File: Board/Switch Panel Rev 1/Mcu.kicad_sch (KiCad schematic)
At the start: 26 parts, among them J4 Conn_ARM_SWD_TagConnect_TC203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, J4 USB_C_Receptacle_USB2.0, U17 STM32G491CEUx, U6 MB85RS64, Y2 32.768kHz, Y3 8MHz

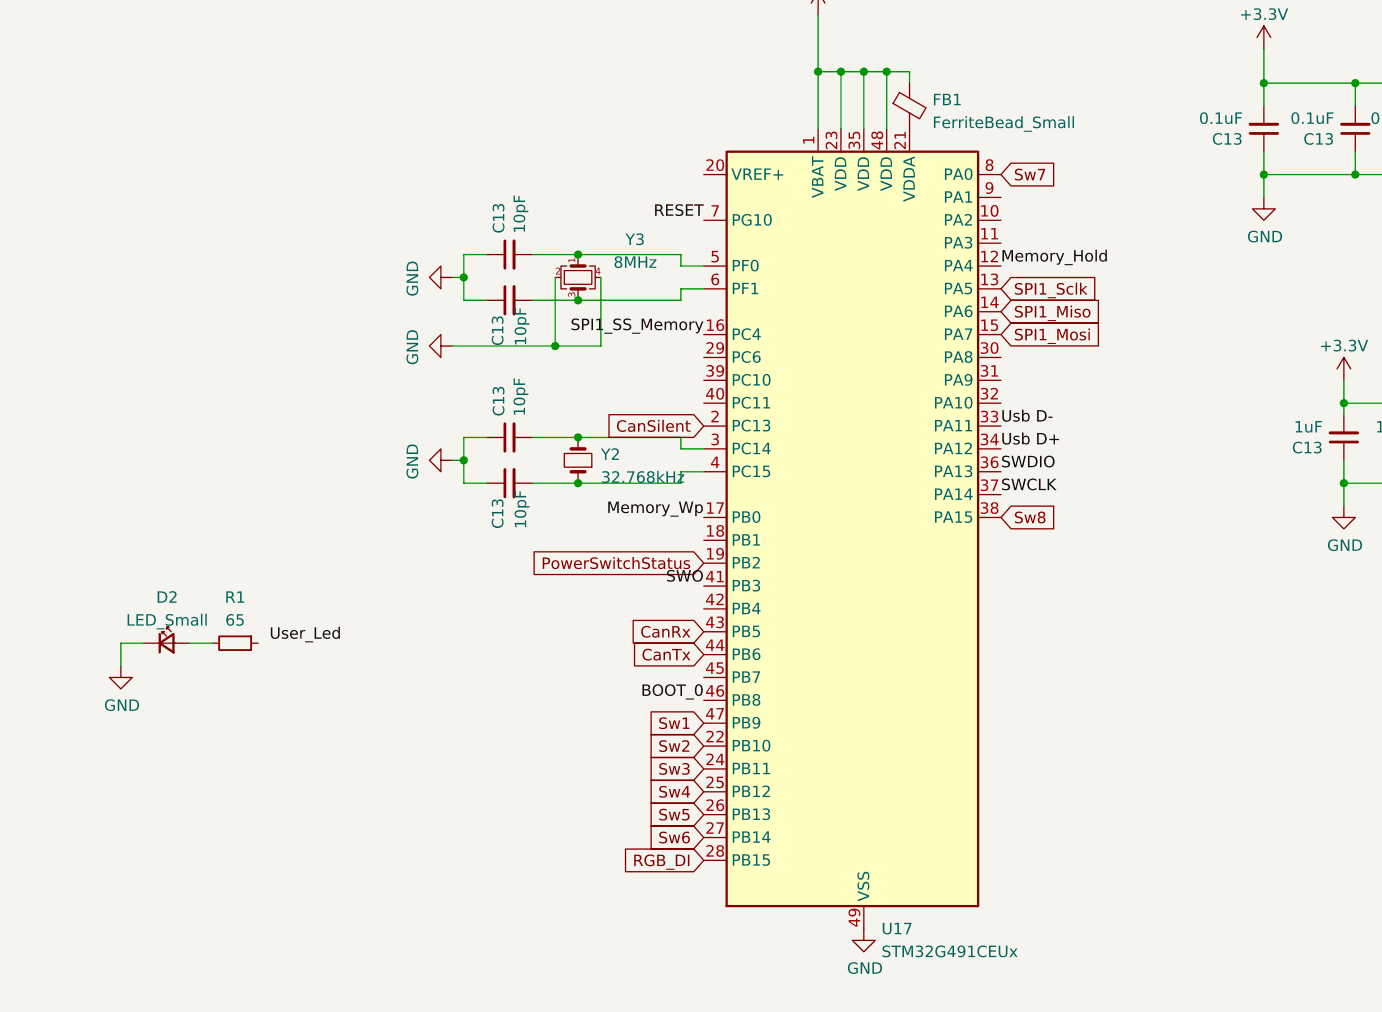
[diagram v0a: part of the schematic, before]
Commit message: Board Updates
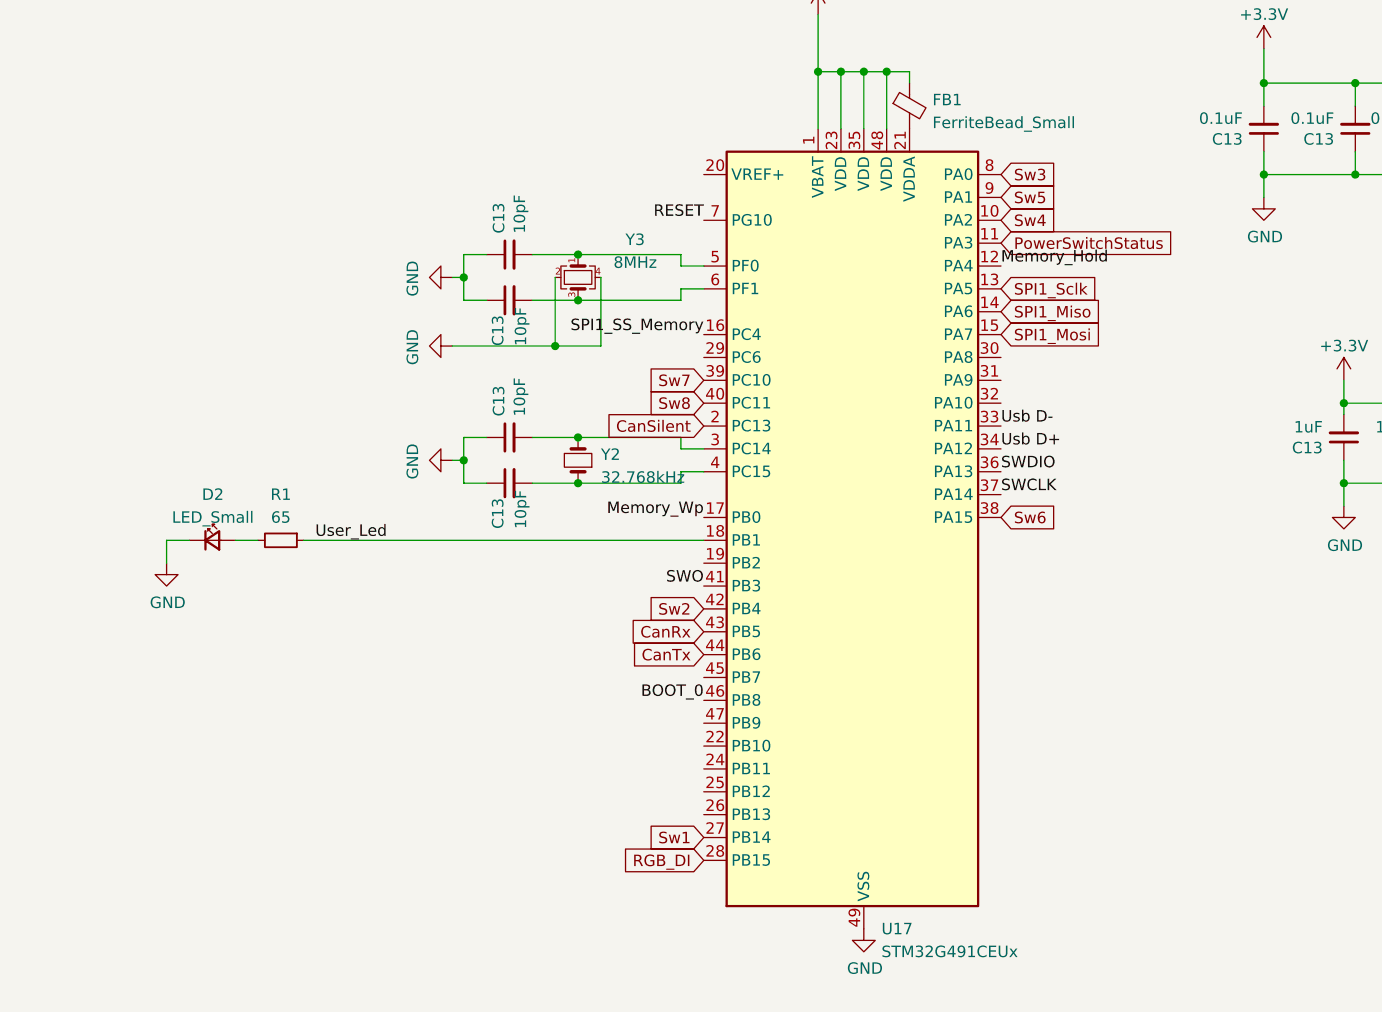
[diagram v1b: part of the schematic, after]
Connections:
- net PowerSwitchStatus: now also U17.11 (PA3); no longer U17.19 (PB2)
- net Sw1: now also U17.27 (PB14); no longer U17.47 (PB9)
- net Sw2: now also U17.42 (PB4); no longer U17.22 (PB10)
- net Sw3: now also U17.8 (PA0); no longer U17.24 (PB11)
- net Sw4: now also U17.10 (PA2); no longer U17.25 (PB12)
- net Sw5: now also U17.9 (PA1); no longer U17.26 (PB13)
- net Sw6: now also U17.38 (PA15); no longer U17.27 (PB14)
- net Sw7: now also U17.39 (PC10); no longer U17.8 (PA0)
- net Sw8: now also U17.40 (PC11); no longer U17.38 (PA15)
- net User_Led: now also R1.1, U17.18 (PB1)
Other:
- moved on the sheet: D2, R1
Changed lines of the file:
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@@
+    (stroke (width 0) (type default))
+  )
+  (wire (pts (xy 40.64 81.28) (xy 85.09 81.28))
     (stroke (width 0) (type default))
   )
@@
     (stroke (width 0) (type default))
   )
-  (wire (pts (xy 22.86 92.71) (xy 20.32 92.71))
+  (wire (pts (xy 27.94 81.28) (xy 25.4 81.28))
     (stroke (width 0) (type default))
   )
@@
     (stroke (width 0) (type default))
   )
-  (wire (pts (xy 27.94 92.71) (xy 30.48 92.71))
+  (wire (pts (xy 33.02 81.28) (xy 35.56 81.28))
     (stroke (width 0) (type default))
   )
@@
     (stroke (width 0) (type default))
   )
-  (wire (pts (xy 20.32 92.71) (xy 20.32 95.25))
+  (wire (pts (xy 25.4 81.28) (xy 25.4 83.82))
     (stroke (width 0) (type default))
   )
@@
     (effects (font (size 1.27 1.27)) (justify right bottom))
   )
-  (label "User_Led" (at 36.83 92.71 0) (fields_autoplaced)
+  (label "User_Led" (at 41.91 81.28 0) (fields_autoplaced)
     (effects (font (size 1.27 1.27)) (justify left bottom))
   )
@@
     (effects (font (size 1.27 1.27)) (justify right bottom))
   )
-  (global_label "Sw8" (shape input) (at 118.11 78.74 0) (fields_autoplaced)
-    (effects (font (size 1.27 1.27)) (justify left))
-    (property "Intersheetrefs" "${INTERSHEET_REFS}" (at 124.7653 78.74 0)
-      (effects (font (size 1.27 1.27)) (justify left) hide)
+  (global_label "Sw8" (shape input) (at 85.09 66.04 180) (fields_autoplaced)
+    (effects (font (size 1.27 1.27)) (justify right))
+    (property "Intersheetrefs" "${INTERSHEET_REFS}" (at 78.4347 66.04 0)
+      (effects (font (size 1.27 1.27)) (justify right) hide)
     )
   )
@@
     )
   )
-  (global_label "Sw6" (shape input) (at 85.09 114.3 180) (fields_autoplaced)
-    (effects (font (size 1.27 1.27)) (justify right))
-    (property "Intersheetrefs" "${INTERSHEET_REFS}" (at 78.4347 114.3 0)
-      (effects (font (size 1.27 1.27)) (justify right) hide)
+  (global_label "Sw6" (shape input) (at 118.11 78.74 0) (fields_autoplaced)
+    (effects (font (size 1.27 1.27)) (justify left))
+    (property "Intersheetrefs" "${INTERSHEET_REFS}" (at 124.7653 78.74 0)
+      (effects (font (size 1.27 1.27)) (justify left) hide)
     )
   )
@@
     )
   )
-  (global_label "Sw2" (shape input) (at 85.09 104.14 180) (fields_autoplaced)
+  (global_label "Sw2" (shape input) (at 85.09 88.9 180) (fields_autoplaced)
     (effects (font (size 1.27 1.27)) (justify right))
-    (property "Intersheetrefs" "${INTERSHEET_REFS}" (at 78.4347 104.14 0)
+    (property "Intersheetrefs" "${INTERSHEET_REFS}" (at 78.4347 88.9 0)
       (effects (font (size 1.27 1.27)) (justify right) hide)
     )
   )
-  (global_label "PowerSwitchStatus" (shape input) (at 85.09 83.82 180) (fields_autoplaced)
+  (global_label "PowerSwitchStatus" (shape input) (at 118.11 48.26 0) (fields_autoplaced)
+    (effects (font (size 1.27 1.27)) (justify left))
+    (property "Intersheetrefs" "${INTERSHEET_REFS}" (at 138.7352 48.26 0)
+      (effects (font (size 1.27 1.27)) (justify left) hide)
+    )
+  )
+  (global_label "Sw1" (shape input) (at 85.09 114.3 180) (fields_autoplaced)
     (effects (font (size 1.27 1.27)) (justify right))
-    (property "Intersheetrefs" "${INTERSHEET_REFS}" (at 64.4648 83.82 0)
-      (effects (font (size 1.27 1.27)) (justify right) hide)
-    )
-  )
-  (global_label "Sw1" (shape input) (at 85.09 101.6 180) (fields_autoplaced)
-    (effects (font (size 1.27 1.27)) (justify right))
-    (property "Intersheetrefs" "${INTERSHEET_REFS}" (at 78.4347 101.6 0)
+    (property "Intersheetrefs" "${INTERSHEET_REFS}" (at 78.4347 114.3 0)
       (effects (font (size 1.27 1.27)) (justify right) hide)
     )
@@
     )
   )
-  (global_label "Sw3" (shape input) (at 85.09 106.68 180) (fields_autoplaced)
-    (effects (font (size 1.27 1.27)) (justify right))
-    (property "Intersheetrefs" "${INTERSHEET_REFS}" (at 78.4347 106.68 0)
-      (effects (font (size 1.27 1.27)) (justify right) hide)
-    )
-  )
-  (global_label "Sw5" (shape input) (at 85.09 111.76 180) (fields_autoplaced)
-    (effects (font (size 1.27 1.27)) (justify right))
-    (property "Intersheetrefs" "${INTERSHEET_REFS}" (at 78.4347 111.76 0)
-      (effects (font (size 1.27 1.27)) (justify right) hide)
-    )
-  )
-  (global_label "Sw4" (shape input) (at 85.09 109.22 180) (fields_autoplaced)
-    (effects (font (size 1.27 1.27)) (justify right))
-    (property "Intersheetrefs" "${INTERSHEET_REFS}" (at 78.4347 109.22 0)
-      (effects (font (size 1.27 1.27)) (justify right) hide)
+  (global_label "Sw3" (shape input) (at 118.11 40.64 0) (fields_autoplaced)
+    (effects (font (size 1.27 1.27)) (justify left))
+    (property "Intersheetrefs" "${INTERSHEET_REFS}" (at 124.7653 40.64 0)
+      (effects (font (size 1.27 1.27)) (justify left) hide)
+    )
+  )
+  (global_label "Sw5" (shape input) (at 118.11 43.18 0) (fields_autoplaced)
+    (effects (font (size 1.27 1.27)) (justify left))
+    (property "Intersheetrefs" "${INTERSHEET_REFS}" (at 124.7653 43.18 0)
+      (effects (font (size 1.27 1.27)) (justify left) hide)
+    )
+  )
+  (global_label "Sw4" (shape input) (at 118.11 45.72 0) (fields_autoplaced)
+    (effects (font (size 1.27 1.27)) (justify left))
+    (property "Intersheetrefs" "${INTERSHEET_REFS}" (at 124.7653 45.72 0)
+      (effects (font (size 1.27 1.27)) (justify left) hide)
     )
   )
@@
     )
   )
-  (global_label "Sw7" (shape input) (at 118.11 40.64 0) (fields_autoplaced)
-    (effects (font (size 1.27 1.27)) (justify left))
-    (property "Intersheetrefs" "${INTERSHEET_REFS}" (at 124.7653 40.64 0)
-      (effects (font (size 1.27 1.27)) (justify left) hide)
+  (global_label "Sw7" (shape input) (at 85.09 63.5 180) (fields_autoplaced)
+    (effects (font (size 1.27 1.27)) (justify right))
+    (property "Intersheetrefs" "${INTERSHEET_REFS}" (at 78.4347 63.5 0)
+      (effects (font (size 1.27 1.27)) (justify right) hide)
     )
   )
@@
     )
   )
-  (symbol (lib_id "power:GND") (at 20.32 95.25 0) (unit 1)
-    (in_bom yes) (on_board yes) (dnp no)
-    (property "Reference" "#PWR018" (at 20.32 101.6 0)
-      (effects (font (size 1.27 1.27)) hide)
-    )
-    (property "Value" "GND" (at 20.447 99.6442 0)
-      (effects (font (size 1.27 1.27)))
-    )
-    (property "Footprint" "" (at 20.32 95.25 0)
-      (effects (font (size 1.27 1.27)) hide)
-    )
-    (property "Datasheet" "" (at 20.32 95.25 0)
+  (symbol (lib_id "power:GND") (at 25.4 83.82 0) (unit 1)
+    (in_bom yes) (on_board yes) (dnp no)
+    (property "Reference" "#PWR018" (at 25.4 90.17 0)
+      (effects (font (size 1.27 1.27)) hide)
+    )
+    (property "Value" "GND" (at 25.527 88.2142 0)
+      (effects (font (size 1.27 1.27)))
+    )
+    (property "Footprint" "" (at 25.4 83.82 0)
+      (effects (font (size 1.27 1.27)) hide)
+    )
+    (property "Datasheet" "" (at 25.4 83.82 0)
       (effects (font (size 1.27 1.27)) hide)
     )
@@
     )
   )
-  (symbol (lib_id "Device:R_Small") (at 33.02 92.71 270) (unit 1)
+  (symbol (lib_id "Device:R_Small") (at 38.1 81.28 270) (unit 1)
     (in_bom yes) (on_board yes) (dnp no) (fields_autoplaced)
-    (property "Reference" "R1" (at 33.02 87.63 90)
-      (effects (font (size 1.27 1.27)))
-    )
-    (property "Value" "65" (at 33.02 90.17 90)
-      (effects (font (size 1.27 1.27)))
-    )
-    (property "Footprint" "Resistor_SMD:R_0603_1608Metric_Pad0.98x0.95mm_HandSolder" (at 33.02 92.71 0)
-      (effects (font (size 1.27 1.27)) hide)
-    )
-    (property "Datasheet" "~" (at 33.02 92.71 0)
+    (property "Reference" "R1" (at 38.1 76.2 90)
+      (effects (font (size 1.27 1.27)))
+    )
+    (property "Value" "65" (at 38.1 78.74 90)
+      (effects (font (size 1.27 1.27)))
+    )
+    (property "Footprint" "Resistor_SMD:R_0603_1608Metric_Pad0.98x0.95mm_HandSolder" (at 38.1 81.28 0)
+      (effects (font (size 1.27 1.27)) hide)
+    )
+    (property "Datasheet" "~" (at 38.1 81.28 0)
       (effects (font (size 1.27 1.27)) hide)
     )
@@
     )
   )
-  (symbol (lib_id "Device:LED_Small") (at 25.4 92.71 0) (unit 1)
+  (symbol (lib_id "Device:LED_Small") (at 30.48 81.28 0) (unit 1)
     (in_bom yes) (on_board yes) (dnp no) (fields_autoplaced)
-    (property "Reference" "D2" (at 25.4635 87.63 0)
-      (effects (font (size 1.27 1.27)))
-    )
-    (property "Value" "LED_Small" (at 25.4635 90.17 0)
-      (effects (font (size 1.27 1.27)))
-    )
-    (property "Footprint" "LED_SMD:LED_0603_1608Metric_Pad1.05x0.95mm_HandSolder" (at 25.4 92.71 90)
-      (effects (font (size 1.27 1.27)) hide)
-    )
-    (property "Datasheet" "~" (at 25.4 92.71 90)
-      (effects (font (size 1.27 1.27)) hide)
-    )
-    (property "Part Number" "150060VS75000 " (at 25.4 92.71 0)
-      (effects (font (size 1.27 1.27)) hide)
-    )
+    (property "Reference" "D2" (at 30.5435 76.2 0)
+      (effects (font (size 1.27 1.27)))
+    )
+    (property "Value" "LED_Small" (at 30.5435 78.74 0)
+      (effects (font (size 1.27 1.27)))
+    )
+    (property "Footprint" "LED_SMD:LED_0603_1608Metric_Pad1.05x0.95mm_HandSolder" (at 30.48 81.28 90)
+      (effects (font (size 1.27 1.27)) hide)
+    )
+    (property "Datasheet" "~" (at 30.48 81.28 90)
+      (effects (font (size 1.27 1.27)) hide)
+    )
+    (property "Part Number" "150060VS75000 " (at 30.48 81.28 0)
+      (effects (font (size 1.27 1.27)) hide)
+    )
